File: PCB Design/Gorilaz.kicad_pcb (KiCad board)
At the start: 2 copper layers, 100 x 86 mm, 50 parts, among them J1 Conn_01x13, J2 Conn_01x13, J3 Conn_01x13, J4 Conn_01x13, J5 HRO_TYPE-C-31-M-14, J6 Battery, J7 Conn_01x13, J8 Conn_01x13, M1 MountingHole_6.4mm_M6, M3 MountingHole_4.3mm_M4, M4 MountingHole_4.3mm_M4, SW4 RST, U1 SRV05-4, U10 MAX17048, U3 BQ24075, U4 DW01A, U5 FS8205, U8 nRF52840_moko_mk08

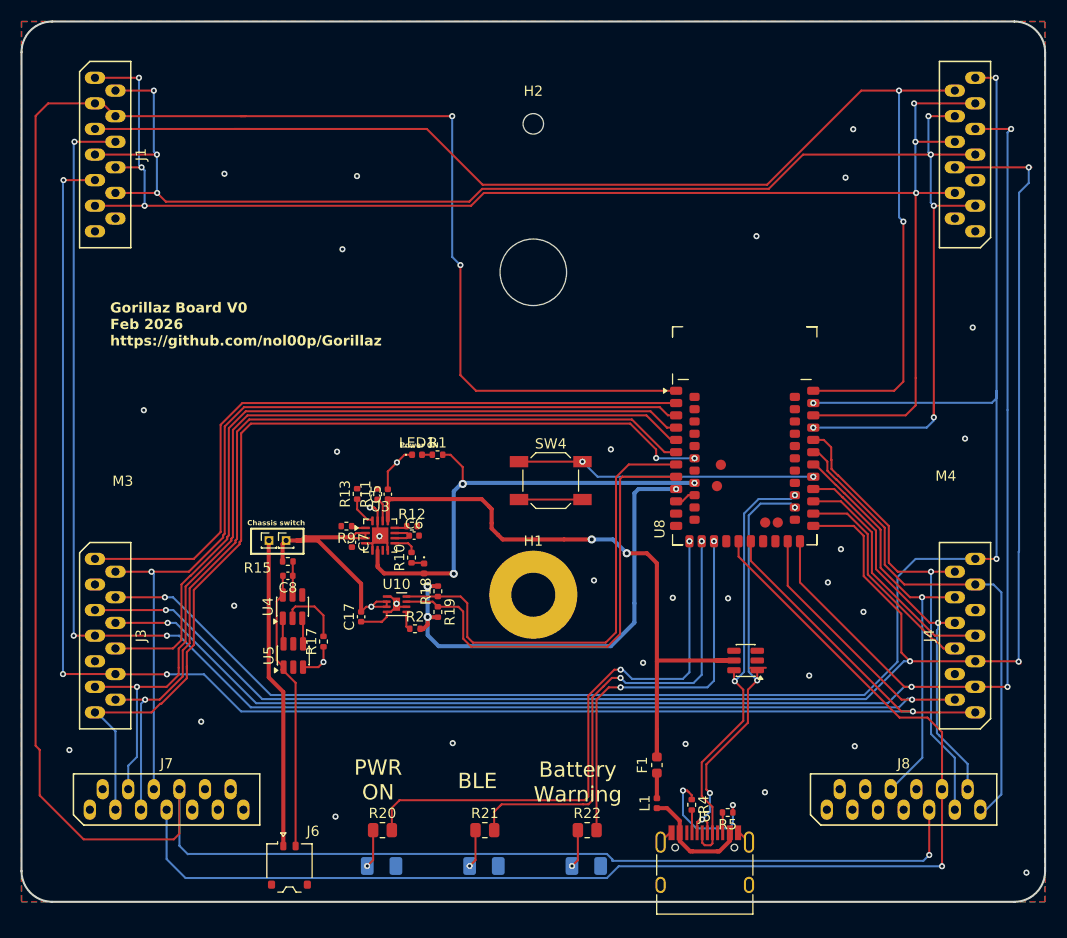
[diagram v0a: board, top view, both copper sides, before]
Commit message: render update
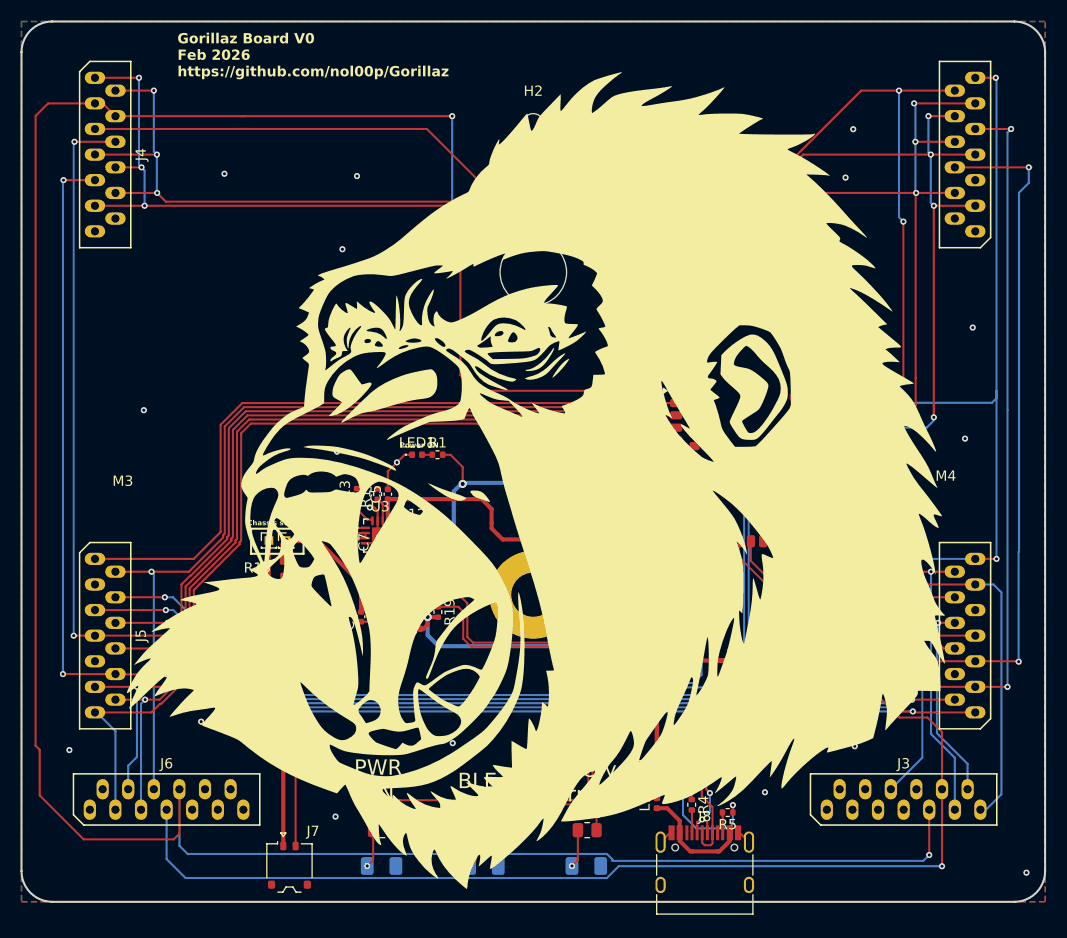
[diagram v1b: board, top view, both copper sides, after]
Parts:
- added G***: LOGO, Local:gorillaz2, F.Cu at (156.4, 84.2)
- renumbered J2 to J1, J4 to J2, J8 to J3, J1 to J4, J3 to J5, J7 to J6, J6 to J7, J5 to J8
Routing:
- net Net-(J7-Pin_1): track 30.2 -> 0.00 mm
- net +BATT: track 27.8 -> 58.0 mm

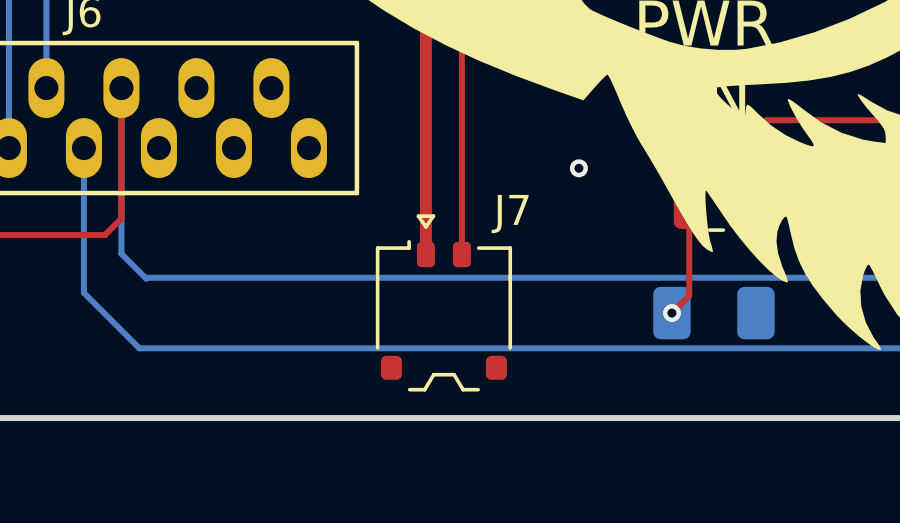
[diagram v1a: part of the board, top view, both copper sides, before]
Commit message: up
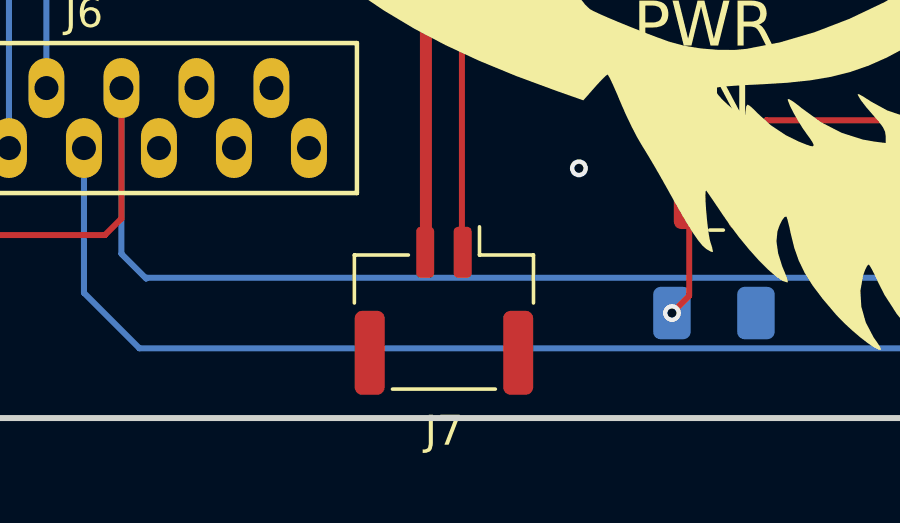
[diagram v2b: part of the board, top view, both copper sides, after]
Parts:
- J7: footprint Local:Molex_Pico-EZmate_78171-0002_1x02-1MP_P1.20mm_Vertical -> Connector_JST:JST_GH_BM02B-GHS-TBT_1x02-1MP_P1.25mm_Vertical
- turned J7 to 180 degrees
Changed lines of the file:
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@@
 			)
 		)
+		(model "/home/skullbocks/Documents/Kicad/3D Lib/Molex_039532135.stp"
+			(offset
+				(xyz -0.5 -2.5 2.5)
+			)
+			(scale
+				(xyz 1 1 1)
+			)
+			(rotate
+				(xyz -0 -0 -0)
+			)
+		)
 	)
 	(footprint "Capacitor_SMD:C_0402_1005Metric"
@@
 		)
 	)
-	(footprint "Local:Molex_Pico-EZmate_78171-0002_1x02-1MP_P1.20mm_Vertical"
+	(footprint "Connector_JST:JST_GH_BM02B-GHS-TBT_1x02-1MP_P1.25mm_Vertical"
 		(layer "F.Cu")
-		(at 132.325 121.625)
-		(descr "Molex Pico-EZmate series connector, 78171-0002 (http://www.molex.com/pdm_docs/sd/781710002_sd.pdf), generated with kicad-footprint-generator")
-		(tags "connector Molex Pico-EZmate side entry")
+		(at 132.325 121.625 180)
+		(descr "JST GH series connector, BM02B-GHS-TBT (http://www.jst-mfg.com/product/pdf/eng/eGH.pdf), generated with kicad-footprint-generator")
+		(tags "connector JST GH vertical")
 		(property "Reference" "J7"
-			(at 2.3 -3.325 0)
+			(at 0 -4 0)
 			(layer "F.SilkS")
 			(effects
@@
 		)
 		(property "Value" "Battery"
-			(at -5.625 1.775 0)
+			(at 0 4 0)
 			(layer "F.Fab")
 			(effects
@@
 		)
 		(property "LCSC" "C505023"
-			(at 0 0 0)
+			(at 0 0 180)
 			(unlocked yes)
 			(layer "F.Fab")
@@
 		(attr smd)
 		(fp_line
-			(start -2.21 -2.09)
-			(end -1.16 -2.09)
+			(start 2.985 1.86)
+			(end 1.185 1.86)
 			(stroke
 				(width 0.12)
@@
 		)
 		(fp_line
-			(start -2.21 1.24)
-			(end -2.21 -2.09)
+			(start 2.985 0.26)
+			(end 2.985 1.86)
 			(stroke
 				(width 0.12)
@@
 		)
 		(fp_line
-			(start -1.16 -2.09)
-			(end -1.16 -2.3)
+			(start -1.185 1.86)
+			(end -1.185 2.8)
 			(stroke
 				(width 0.12)
@@
 		)
 		(fp_line
-			(start -1.14 2.63)
-			(end -0.64 2.63)
+			(start -1.715 -2.61)
+			(end 1.715 -2.61)
 			(stroke
 				(width 0.12)
@@
 		)
 		(fp_line
-			(start -0.85 -3.153553)
-			(end -0.6 -2.8)
+			(start -2.985 1.86)
+			(end -1.185 1.86)
 			(stroke
 				(width 0.12)
@@
 		)
 		(fp_line
-			(start -0.64 2.63)
-			(end -0.34 2.13)
+			(start -2.985 0.26)
+			(end -2.985 1.86)
 			(stroke
 				(width 0.12)
@@
 		)
 		(fp_line
-			(start -0.6 -2.8)
-			(end -0.35 -3.153553)
+			(start 3.48 0.5)
+			(end 3.38 0.5)
 			(stroke
-				(width 0.12)
+				(width 0.05)
 				(type solid)
 			)
-			(layer "F.SilkS")
+			(layer "F.CrtYd")
 		)
 		(fp_line
-			(start -0.35 -3.153553)
-			(end -0.85 -3.153553)
+			(start 3.48 -3.3)
+			(end 3.48 0.5)
 			(stroke
-				(width 0.12)
+				(width 0.05)
 				(type solid)
 			)
-			(layer "F.SilkS")
+			(layer "F.CrtYd")
 		)
 		(fp_line
-			(start -0.34 2.13)
-			(end 0.34 2.13)
+			(start 3.38 2.25)
+			(end 1.43 2.25)
 			(stroke
-				(width 0.12)
+				(width 0.05)
 				(type solid)
 			)
-			(layer "F.SilkS")
+			(layer "F.CrtYd")
 		)
 		(fp_line
-			(start 0.34 2.13)
-			(end 0.64 2.63)
+			(start 3.38 0.5)
+			(end 3.38 2.25)
 			(stroke
-				(width 0.12)
+				(width 0.05)
 				(type solid)
 			)
-			(layer "F.SilkS")
+			(layer "F.CrtYd")
 		)
 		(fp_line
-			(start 0.64 2.63)
-			(end 1.14 2.63)
+			(start 1.47 -3)
+			(end 1.47 -3.3)
 			(stroke
-				(width 0.12)
+				(width 0.05)
 				(type solid)
 			)
-			(layer "F.SilkS")
+			(layer "F.CrtYd")
 		)
 		(fp_line
-			(start 2.21 -2.09)
-			(end 1.16 -2.09)
+			(start 1.47 -3.3)
+			(end 3.48 -3.3)
 			(stroke
-				(width 0.12)
+				(width 0.05)
 				(type solid)
 			)
-			(layer "F.SilkS")
+			(layer "F.CrtYd")
 		)
 		(fp_line
-			(start 2.21 1.24)
-			(end 2.21 -2.09)
+			(start 1.43 3.3)
+			(end -1.43 3.3)
 			(stroke
-				(width 0.12)
+				(width 0.05)
 				(type solid)
 			)
-			(layer "F.SilkS")
+			(layer "F.CrtYd")
 		)
 		(fp_line
-			(start -2.6 -2.8)
-			(end -2.6 3.02)
+			(start 1.43 2.25)
+			(end 1.43 3.3)
 			(stroke
 				(width 0.05)
@@
 		)
 		(fp_line
-			(start -2.6 3.02)
-			(end 2.6 3.02)
+			(start -1.43 3.3)
+			(end -1.43 2.25)
 			(stroke
 				(width 0.05)
@@
 		)
 		(fp_line
-			(start 2.6 -2.8)
-			(end -2.6 -2.8)
+			(start -1.43 2.25)
+			(end -3.38 2.25)
 			(stroke
 				(width 0.05)
@@
 		)
 		(fp_line
-			(start 2.6 3.02)
-			(end 2.6 -2.8)
+			(start -1.47 -3)
+			(end 1.47 -3)
 			(stroke
 				(width 0.05)
@@
 		)
 		(fp_line
-			(start -2.1 -1.98)
-			(end -2.1 2.52)
+			(start -1.47 -3.3)
+			(end -1.47 -3)
 			(stroke
-				(width 0.1)
+				(width 0.05)
 				(type solid)
 			)
-			(layer "F.Fab")
+			(layer "F.CrtYd")
 		)
 		(fp_line
-			(start -2.1 -1.98)
-			(end 2.1 -1.98)
+			(start -3.38 2.25)
+			(end -3.38 0.5)
 			(stroke
-				(width 0.1)
+				(width 0.05)
 				(type solid)
 			)
-			(layer "F.Fab")
+			(layer "F.CrtYd")
 		)
 		(fp_line
-			(start -2.1 2.52)
-			(end -0.75 2.52)
+			(start -3.38 0.5)
+			(end -3.48 0.5)
+			(stroke
+				(width 0.05)
+				(type solid)
+			)
+			(layer "F.CrtYd")
+		)
+		(fp_line
+			(start -3.48 0.5)
+			(end -3.48 -3.3)
+			(stroke
+				(width 0.05)
+				(type solid)
+			)
+			(layer "F.CrtYd")
+		)
+		(fp_line
+			(start -3.48 -3.3)
+			(end -1.47 -3.3)
+			(stroke
+				(width 0.05)
+				(type solid)
+			)
+			(layer "F.CrtYd")
+		)
+		(fp_line
+			(start 2.875 1.75)
+			(end 2.875 -2.5)
 			(stroke
 				(width 0.1)
@@
 		)
 		(fp_line
-			(start -1.1 -1.98)
-			(end -0.6 -1.272893)
+			(start -0.625 1.042893)
+			(end -0.125 1.75)
 			(stroke
 				(width 0.1)
@@
 		)
 		(fp_line
-			(start -0.75 2.52)
-			(end -0.45 2.02)
+			(start -1.125 1.75)
+			(end -0.625 1.042893)
 			(stroke
 				(width 0.1)
@@
 		)
 		(fp_line
-			(start -0.6 -1.272893)
-			(end -0.1 -1.98)
+			(start -2.875 1.75)
+			(end 2.875 1.75)
 			(stroke
 				(width 0.1)
@@
 		)
 		(fp_line
-			(start -0.45 2.02)
-			(end 0.45 2.02)
+			(start -2.875 1.75)
+			(end -2.875 -2.5)
 			(stroke
 				(width 0.1)
@@
 		)
 		(fp_line
-			(start 0.45 2.02)
-			(end 0.75 2.52)
+			(start -2.875 -2.5)
+			(end 2.875 -2.5)
 			(stroke
 				(width 0.1)
@@
 			(layer "F.Fab")
 		)
-		(fp_line
-			(start 0.75 2.52)
-			(end 2.1 2.52)
+		(fp_rect
+			(start 0.375 -0.5)
+			(end 0.875 0)
 			(stroke
 				(width 0.1)
 				(type solid)
 			)
+			(fill no)
 			(layer "F.Fab")
 		)
-		(fp_line
-			(start 2.1 -1.98)
-			(end 2.1 2.52)
+		(fp_rect
+			(start -0.875 -0.5)
+			(end -0.375 0)
 			(stroke
 				(width 0.1)
 				(type solid)
 			)
+			(fill no)
 			(layer "F.Fab")
 		)
 		(fp_text user "${REFERENCE}"
-			(at 0 0.27 0)
+			(at 0 -1.5 0)
 			(layer "F.Fab")
 			(effects
@@
 		)
 		(pad "1" smd roundrect
-			(at -0.6 -1.875)
-			(size 0.6 0.85)
+			(at -0.625 1.95 180)
+			(size 0.6 1.7)
 			(layers "F.Cu" "F.Mask" "F.Paste")
 			(roundrect_rratio 0.25)
@@
 		)
 		(pad "2" smd roundrect
-			(at 0.6 -1.875)
-			(size 0.6 0.85)
+			(at 0.625 1.95 180)
+			(size 0.6 1.7)
 			(layers "F.Cu" "F.Mask" "F.Paste")
 			(roundrect_rratio 0.25)
@@
 		)
 		(pad "MP" smd roundrect
-			(at -1.75 1.9)
-			(size 0.7 0.8)
+			(at -2.475 -1.4 180)
+			(size 1 2.8)
 			(layers "F.Cu" "F.Mask" "F.Paste")
 			(roundrect_rratio 0.25)
@@
 		)
 		(pad "MP" smd roundrect
-			(at 1.75 1.9)
-			(size 0.7 0.8)
+			(at 2.475 -1.4 180)
+			(size 1 2.8)
 			(layers "F.Cu" "F.Mask" "F.Paste")
 			(roundrect_rratio 0.25)
@@
 		)
 		(embedded_fonts no)
-		(model "${KISYS3DMOD}/Connector_Molex.3dshapes/Molex_Pico-EZmate_78171-0002_1x02-1MP_P1.20mm_Vertical.wrl"
+		(model "${KICAD9_3DMODEL_DIR}/Connector_JST.3dshapes/JST_GH_BM02B-GHS-TBT_1x02-1MP_P1.25mm_Vertical.step"
 			(offset
 				(xyz 0 0 0)
